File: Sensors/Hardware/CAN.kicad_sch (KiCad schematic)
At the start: 11 parts, among them U4 SN65HVD230

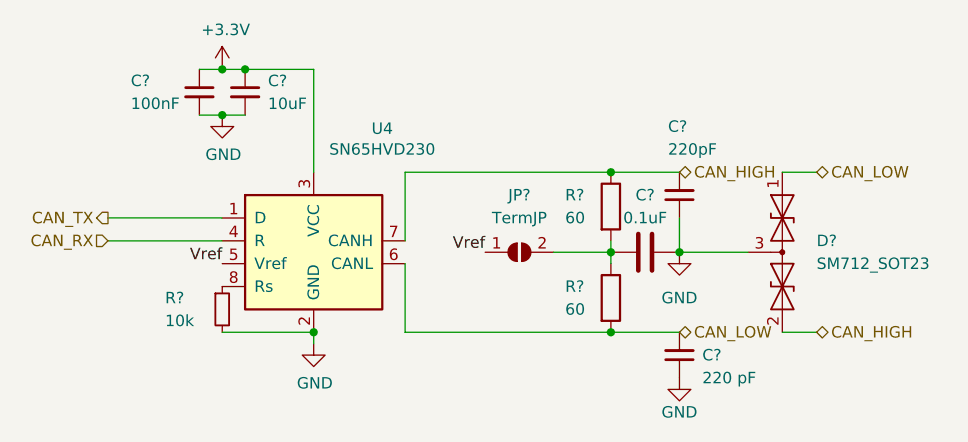
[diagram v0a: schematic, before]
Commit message: fixed hierarchical labels and added ref values
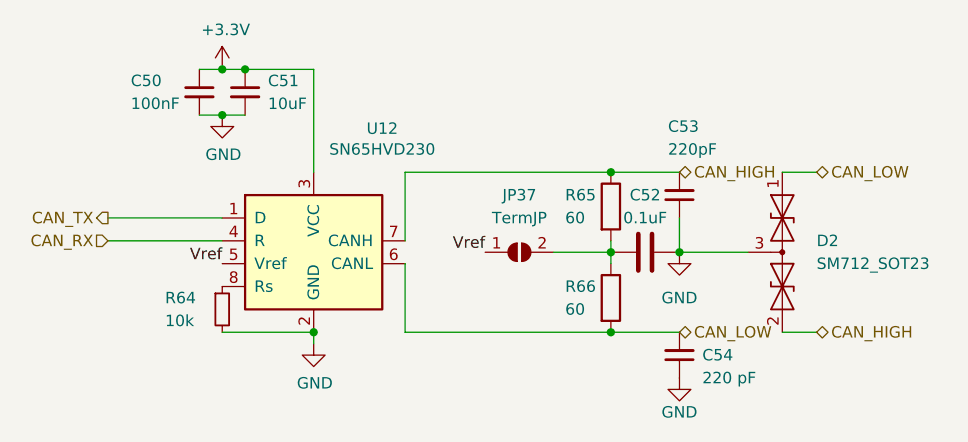
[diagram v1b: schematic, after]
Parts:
- gave numbers to parts that had none: 10
- renumbered U4 to U12
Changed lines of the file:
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@@
   (symbol (lib_id "power:GND") (at 134.62 99.06 0) (unit 1)
     (in_bom yes) (on_board yes) (fields_autoplaced)
-    (property "Reference" "#PWR?" (id 0) (at 134.62 105.41 0)
+    (property "Reference" "#PWR0139" (id 0) (at 134.62 105.41 0)
       (effects (font (size 1.27 1.27)) hide)
     )
@@
   (symbol (lib_id "power:+3.3V") (at 124.46 68.58 0) (unit 1)
     (in_bom yes) (on_board yes) (fields_autoplaced)
-    (property "Reference" "#PWR?" (id 0) (at 124.46 72.39 0)
+    (property "Reference" "#PWR0137" (id 0) (at 124.46 72.39 0)
       (effects (font (size 1.27 1.27)) hide)
     )
@@
   (symbol (lib_id "Interface_CAN_LIN:SN65HVD230") (at 134.62 87.63 0) (unit 1)
     (in_bom yes) (on_board yes) (fields_autoplaced)
-    (property "Reference" "U?" (id 0) (at 142.24 75.1586 0))
+    (property "Reference" "U12" (id 0) (at 142.24 75.1586 0))
     (property "Value" "SN65HVD230" (id 1) (at 142.24 77.47 0))
     (property "Footprint" "Package_SO:SOIC-8_3.9x4.9mm_P1.27mm" (id 2) (at 134.62 100.33 0)
@@
   (symbol (lib_id "Device:C_Small") (at 127 71.12 0) (unit 1)
     (in_bom yes) (on_board yes) (fields_autoplaced)
-    (property "Reference" "C?" (id 0) (at 129.54 69.8562 0)
+    (property "Reference" "C51" (id 0) (at 129.54 69.8562 0)
       (effects (font (size 1.27 1.27)) (justify left))
     )
@@
   (symbol (lib_id "Device:C_Small") (at 175.26 82.55 180) (unit 1)
     (in_bom yes) (on_board yes)
-    (property "Reference" "C?" (id 0) (at 173.99 74.93 0)
+    (property "Reference" "C53" (id 0) (at 173.99 74.93 0)
       (effects (font (size 1.27 1.27)) (justify right))
     )
@@
   (symbol (lib_id "Diode:SM712_SOT23") (at 186.69 88.9 270) (unit 1)
     (in_bom yes) (on_board yes) (fields_autoplaced)
-    (property "Reference" "D?" (id 0) (at 190.5 87.63 90)
+    (property "Reference" "D2" (id 0) (at 190.5 87.63 90)
       (effects (font (size 1.27 1.27)) (justify left))
     )
@@
   (symbol (lib_id "power:GND") (at 175.26 88.9 0) (unit 1)
     (in_bom yes) (on_board yes) (fields_autoplaced)
-    (property "Reference" "#PWR?" (id 0) (at 175.26 95.25 0)
+    (property "Reference" "#PWR0140" (id 0) (at 175.26 95.25 0)
       (effects (font (size 1.27 1.27)) hide)
     )
@@
   (symbol (lib_id "power:GND") (at 175.26 102.87 0) (unit 1)
     (in_bom yes) (on_board yes) (fields_autoplaced)
-    (property "Reference" "#PWR?" (id 0) (at 175.26 109.22 0)
+    (property "Reference" "#PWR0141" (id 0) (at 175.26 109.22 0)
       (effects (font (size 1.27 1.27)) hide)
     )
@@
   (symbol (lib_id "Device:C_Small") (at 121.92 71.12 0) (unit 1)
     (in_bom yes) (on_board yes) (fields_autoplaced)
-    (property "Reference" "C?" (id 0) (at 114.3 69.85 0)
+    (property "Reference" "C50" (id 0) (at 114.3 69.85 0)
       (effects (font (size 1.27 1.27)) (justify left))
     )
@@
   (symbol (lib_id "Device:R_Small") (at 124.46 95.25 0) (unit 1)
     (in_bom yes) (on_board yes)
-    (property "Reference" "R?" (id 0) (at 118.11 93.98 0)
+    (property "Reference" "R64" (id 0) (at 118.11 93.98 0)
       (effects (font (size 1.27 1.27)) (justify left))
     )
@@
   (symbol (lib_id "Device:R") (at 167.64 93.98 0) (unit 1)
     (in_bom yes) (on_board yes) (fields_autoplaced)
-    (property "Reference" "R?" (id 0) (at 162.56 92.71 0)
+    (property "Reference" "R66" (id 0) (at 162.56 92.71 0)
       (effects (font (size 1.27 1.27)) (justify left))
     )
@@
   (symbol (lib_id "Device:R") (at 167.64 83.82 0) (unit 1)
     (in_bom yes) (on_board yes) (fields_autoplaced)
-    (property "Reference" "R?" (id 0) (at 162.56 82.55 0)
+    (property "Reference" "R65" (id 0) (at 162.56 82.55 0)
       (effects (font (size 1.27 1.27)) (justify left))
     )
@@
   (symbol (lib_id "Device:C") (at 171.45 88.9 90) (unit 1)
     (in_bom yes) (on_board yes) (fields_autoplaced)
-    (property "Reference" "C?" (id 0) (at 171.45 82.55 90))
+    (property "Reference" "C52" (id 0) (at 171.45 82.55 90))
     (property "Value" "0.1uF" (id 1) (at 171.45 85.09 90))
     (property "Footprint" "Capacitor_SMD:C_0402_1005Metric" (id 2) (at 175.26 87.9348 0)
@@
   (symbol (lib_id "power:GND") (at 124.46 73.66 0) (unit 1)
     (in_bom yes) (on_board yes) (fields_autoplaced)
-    (property "Reference" "#PWR?" (id 0) (at 124.46 80.01 0)
+    (property "Reference" "#PWR0138" (id 0) (at 124.46 80.01 0)
       (effects (font (size 1.27 1.27)) hide)
     )
@@
   (symbol (lib_id "Jumper:SolderJumper_2_Open") (at 157.48 88.9 0) (unit 1)
     (in_bom yes) (on_board yes) (fields_autoplaced)
-    (property "Reference" "JP?" (id 0) (at 157.48 82.55 0))
+    (property "Reference" "JP37" (id 0) (at 157.48 82.55 0))
     (property "Value" "TermJP" (id 1) (at 157.48 85.09 0))
     (property "Footprint" "" (id 2) (at 157.48 88.9 0)
@@
   (symbol (lib_id "Device:C_Small") (at 175.26 100.33 180) (unit 1)
     (in_bom yes) (on_board yes) (fields_autoplaced)
-    (property "Reference" "C?" (id 0) (at 177.8 100.33 0)
+    (property "Reference" "C54" (id 0) (at 177.8 100.33 0)
       (effects (font (size 1.27 1.27)) (justify right))
     )

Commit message: added 10V rail, moved to boosts sheet
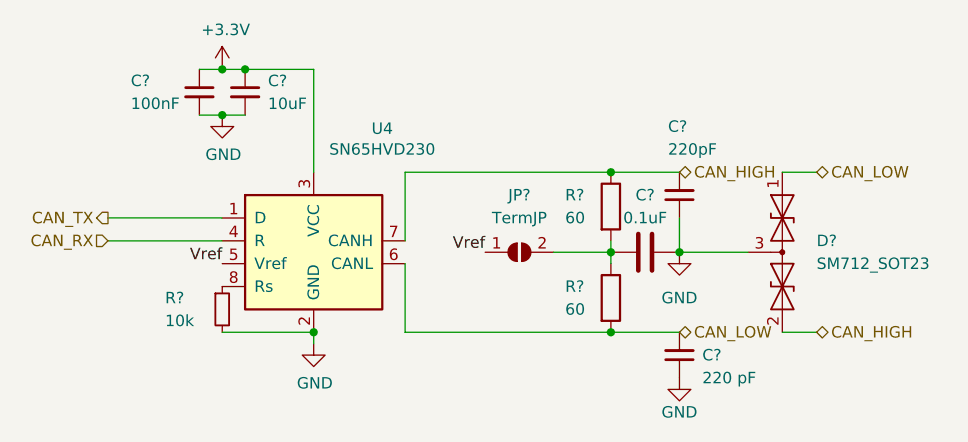
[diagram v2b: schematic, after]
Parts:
- renumbered C51 to C?, C53 to C?, C50 to C?, C52 to C?, C54 to C?, D2 to D?, JP37 to JP?, R64 to R?, R66 to R?, R65 to R?, U12 to U4
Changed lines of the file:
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@@
   (symbol (lib_id "power:GND") (at 134.62 99.06 0) (unit 1)
     (in_bom yes) (on_board yes) (fields_autoplaced)
-    (property "Reference" "#PWR0139" (id 0) (at 134.62 105.41 0)
+    (property "Reference" "#PWR?" (id 0) (at 134.62 105.41 0)
       (effects (font (size 1.27 1.27)) hide)
     )
@@
   (symbol (lib_id "power:+3.3V") (at 124.46 68.58 0) (unit 1)
     (in_bom yes) (on_board yes) (fields_autoplaced)
-    (property "Reference" "#PWR0137" (id 0) (at 124.46 72.39 0)
+    (property "Reference" "#PWR?" (id 0) (at 124.46 72.39 0)
       (effects (font (size 1.27 1.27)) hide)
     )
@@
   (symbol (lib_id "Interface_CAN_LIN:SN65HVD230") (at 134.62 87.63 0) (unit 1)
     (in_bom yes) (on_board yes) (fields_autoplaced)
-    (property "Reference" "U12" (id 0) (at 142.24 75.1586 0))
+    (property "Reference" "U?" (id 0) (at 142.24 75.1586 0))
     (property "Value" "SN65HVD230" (id 1) (at 142.24 77.47 0))
     (property "Footprint" "Package_SO:SOIC-8_3.9x4.9mm_P1.27mm" (id 2) (at 134.62 100.33 0)
@@
   (symbol (lib_id "Device:C_Small") (at 127 71.12 0) (unit 1)
     (in_bom yes) (on_board yes) (fields_autoplaced)
-    (property "Reference" "C51" (id 0) (at 129.54 69.8562 0)
+    (property "Reference" "C?" (id 0) (at 129.54 69.8562 0)
       (effects (font (size 1.27 1.27)) (justify left))
     )
@@
   (symbol (lib_id "Device:C_Small") (at 175.26 82.55 180) (unit 1)
     (in_bom yes) (on_board yes)
-    (property "Reference" "C53" (id 0) (at 173.99 74.93 0)
+    (property "Reference" "C?" (id 0) (at 173.99 74.93 0)
       (effects (font (size 1.27 1.27)) (justify right))
     )
@@
   (symbol (lib_id "Diode:SM712_SOT23") (at 186.69 88.9 270) (unit 1)
     (in_bom yes) (on_board yes) (fields_autoplaced)
-    (property "Reference" "D2" (id 0) (at 190.5 87.63 90)
+    (property "Reference" "D?" (id 0) (at 190.5 87.63 90)
       (effects (font (size 1.27 1.27)) (justify left))
     )
@@
   (symbol (lib_id "power:GND") (at 175.26 88.9 0) (unit 1)
     (in_bom yes) (on_board yes) (fields_autoplaced)
-    (property "Reference" "#PWR0140" (id 0) (at 175.26 95.25 0)
+    (property "Reference" "#PWR?" (id 0) (at 175.26 95.25 0)
       (effects (font (size 1.27 1.27)) hide)
     )
@@
   (symbol (lib_id "power:GND") (at 175.26 102.87 0) (unit 1)
     (in_bom yes) (on_board yes) (fields_autoplaced)
-    (property "Reference" "#PWR0141" (id 0) (at 175.26 109.22 0)
+    (property "Reference" "#PWR?" (id 0) (at 175.26 109.22 0)
       (effects (font (size 1.27 1.27)) hide)
     )
@@
   (symbol (lib_id "Device:C_Small") (at 121.92 71.12 0) (unit 1)
     (in_bom yes) (on_board yes) (fields_autoplaced)
-    (property "Reference" "C50" (id 0) (at 114.3 69.85 0)
+    (property "Reference" "C?" (id 0) (at 114.3 69.85 0)
       (effects (font (size 1.27 1.27)) (justify left))
     )
@@
   (symbol (lib_id "Device:R_Small") (at 124.46 95.25 0) (unit 1)
     (in_bom yes) (on_board yes)
-    (property "Reference" "R64" (id 0) (at 118.11 93.98 0)
+    (property "Reference" "R?" (id 0) (at 118.11 93.98 0)
       (effects (font (size 1.27 1.27)) (justify left))
     )
@@
   (symbol (lib_id "Device:R") (at 167.64 93.98 0) (unit 1)
     (in_bom yes) (on_board yes) (fields_autoplaced)
-    (property "Reference" "R66" (id 0) (at 162.56 92.71 0)
+    (property "Reference" "R?" (id 0) (at 162.56 92.71 0)
       (effects (font (size 1.27 1.27)) (justify left))
     )
@@
   (symbol (lib_id "Device:R") (at 167.64 83.82 0) (unit 1)
     (in_bom yes) (on_board yes) (fields_autoplaced)
-    (property "Reference" "R65" (id 0) (at 162.56 82.55 0)
+    (property "Reference" "R?" (id 0) (at 162.56 82.55 0)
       (effects (font (size 1.27 1.27)) (justify left))
     )
@@
   (symbol (lib_id "Device:C") (at 171.45 88.9 90) (unit 1)
     (in_bom yes) (on_board yes) (fields_autoplaced)
-    (property "Reference" "C52" (id 0) (at 171.45 82.55 90))
+    (property "Reference" "C?" (id 0) (at 171.45 82.55 90))
     (property "Value" "0.1uF" (id 1) (at 171.45 85.09 90))
     (property "Footprint" "Capacitor_SMD:C_0402_1005Metric" (id 2) (at 175.26 87.9348 0)
@@
   (symbol (lib_id "power:GND") (at 124.46 73.66 0) (unit 1)
     (in_bom yes) (on_board yes) (fields_autoplaced)
-    (property "Reference" "#PWR0138" (id 0) (at 124.46 80.01 0)
+    (property "Reference" "#PWR?" (id 0) (at 124.46 80.01 0)
       (effects (font (size 1.27 1.27)) hide)
     )
@@
   (symbol (lib_id "Jumper:SolderJumper_2_Open") (at 157.48 88.9 0) (unit 1)
     (in_bom yes) (on_board yes) (fields_autoplaced)
-    (property "Reference" "JP37" (id 0) (at 157.48 82.55 0))
+    (property "Reference" "JP?" (id 0) (at 157.48 82.55 0))
     (property "Value" "TermJP" (id 1) (at 157.48 85.09 0))
     (property "Footprint" "" (id 2) (at 157.48 88.9 0)
@@
   (symbol (lib_id "Device:C_Small") (at 175.26 100.33 180) (unit 1)
     (in_bom yes) (on_board yes) (fields_autoplaced)
-    (property "Reference" "C54" (id 0) (at 177.8 100.33 0)
+    (property "Reference" "C?" (id 0) (at 177.8 100.33 0)
       (effects (font (size 1.27 1.27)) (justify right))
     )
